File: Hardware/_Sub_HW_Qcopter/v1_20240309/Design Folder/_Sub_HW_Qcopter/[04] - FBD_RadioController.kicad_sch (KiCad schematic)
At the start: 0 parts

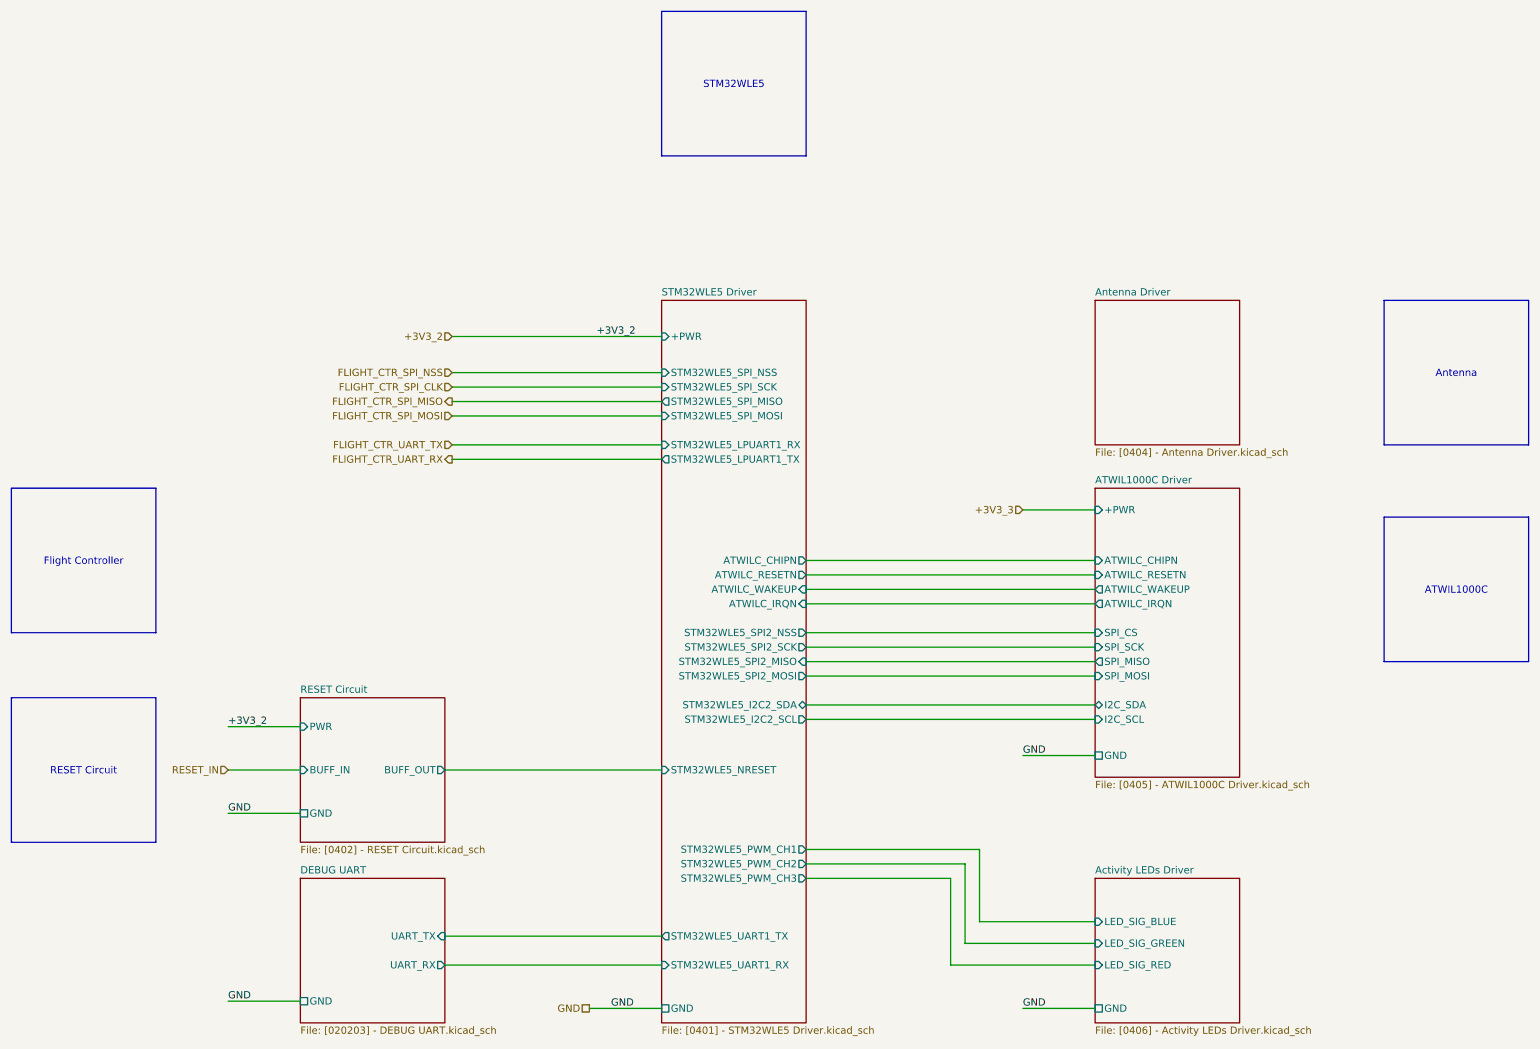
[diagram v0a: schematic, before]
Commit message: 97% drawing schematic is done
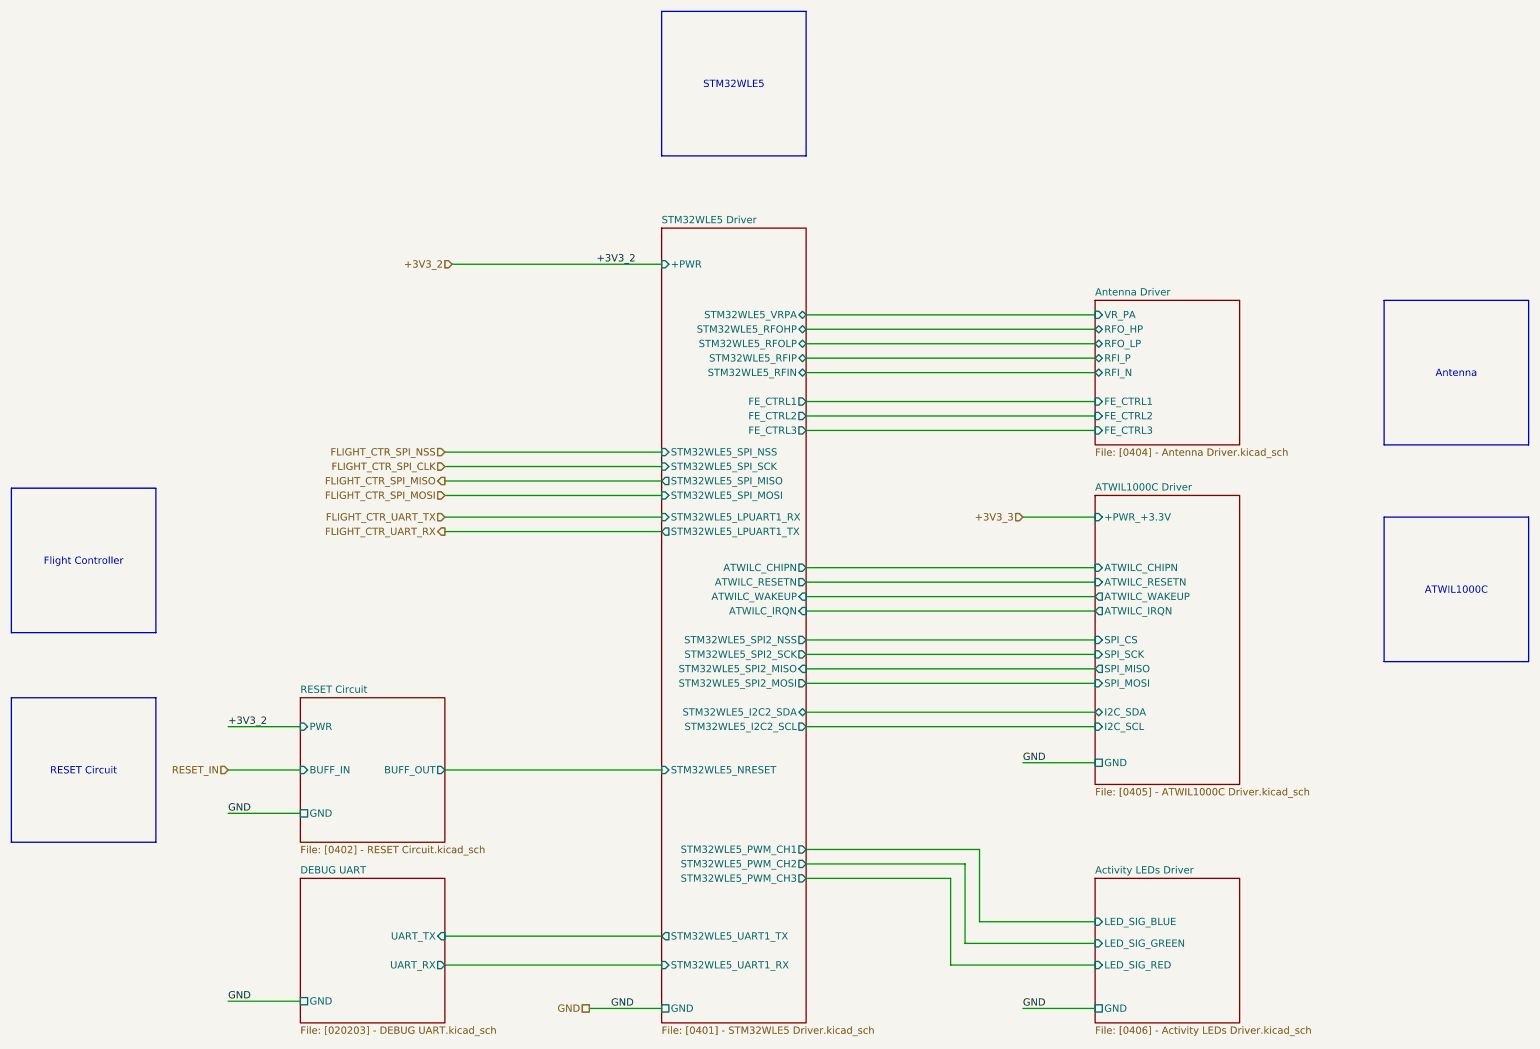
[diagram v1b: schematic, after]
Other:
- sheet ATWIL1000C Driver ports: added +PWR_+3.3V; removed +PWR
- sheet Antenna Driver ports: added FE_CTRL1, FE_CTRL2, FE_CTRL3, RFI_N, RFI_P, RFO_HP, RFO_LP, VR_PA; removed none
- sheet STM32WLE5 Driver ports: added FE_CTRL1, FE_CTRL2, FE_CTRL3, STM32WLE5_RFIN, STM32WLE5_RFIP, STM32WLE5_RFOHP, STM32WLE5_RFOLP, STM32WLE5_VRPA; removed none
